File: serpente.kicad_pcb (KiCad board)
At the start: 2 copper layers, 24 x 22 mm, 31 parts, among them J1 USB_C_Receptacle_USB2.0, J2 Conn_Power, J3 Conn_GPIO, SW1 SW_RESET, U1 GD25Q32CNIGR, U2 MCP1700-3302E_SOT23, U3 ATSAMD21E18A

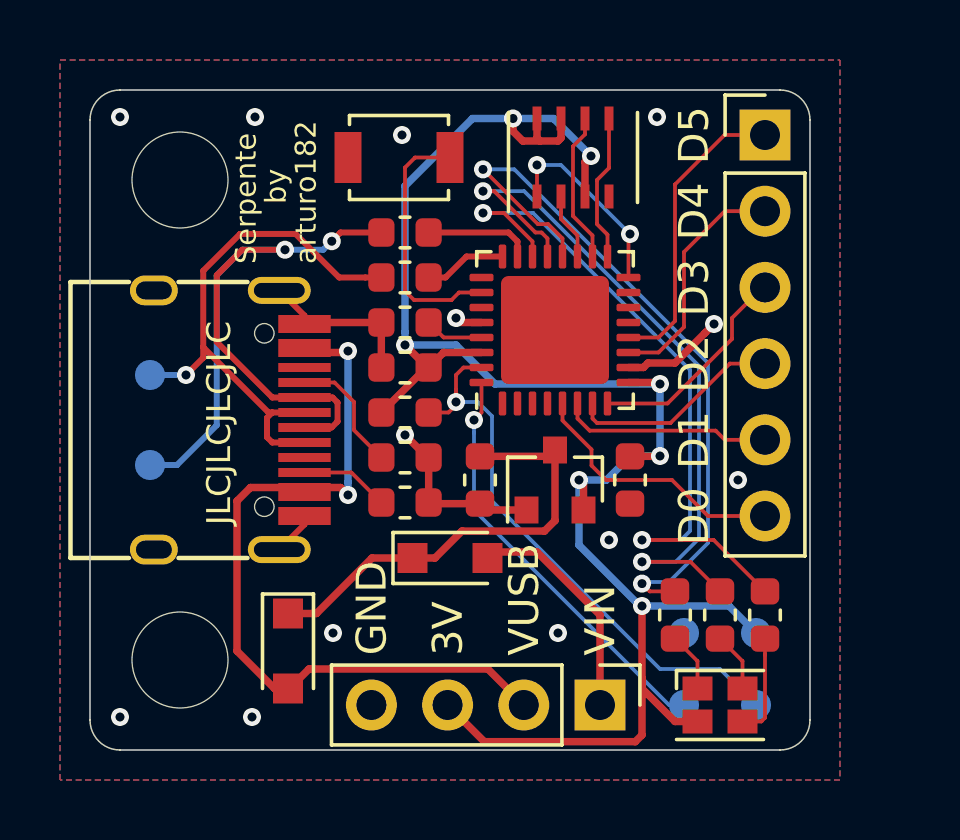
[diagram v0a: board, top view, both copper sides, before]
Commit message: Final rev 2 release!
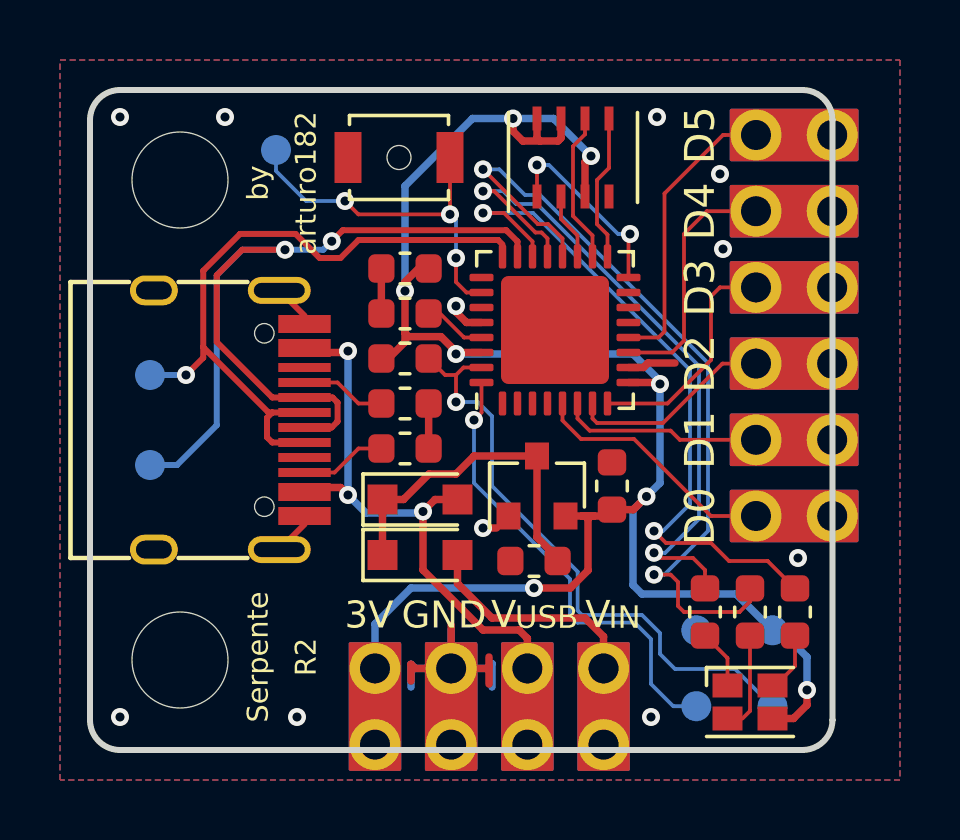
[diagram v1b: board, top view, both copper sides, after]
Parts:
- removed R7, R8: 22R, Resistor_SMD:R_0603_1608Metric
- added TP7: TP_RESET, TestPoint:TestPoint_Pad_D1.0mm, B.Cu at (123.2, 47.0)
- D3: value LED_ARGB -> LED_RBAG
- J2: footprint Connector_PinHeader_2.54mm:PinHeader_1x04_P2.54mm_Vertical -> Connector_PinHeader_2.54mm_Extra:PinHeader_1x04_P2.54mm_Vertical_Castellated
- J3: footprint Connector_PinHeader_2.54mm:PinHeader_1x06_P2.54mm_Vertical -> Connector_PinHeader_2.54mm_Extra:PinHeader_1x06_P2.54mm_Vertical_Castellated
- SW1: footprint Button_Switch_SMD:SW_SPST_B3U-1000P -> Button_Switch_SMD:SW_SPST_B3U-1000P-B
- moved D1 6.70 mm to (128.0, 58.6), turned to 0 degrees
- moved C2 3.30 mm to (127.5, 51.0)
- moved C1 3.24 mm to (131.8, 60.7), turned to 0 degrees
- moved R3 2.50 mm to (140.5, 62.4)
- moved R4 1.80 mm to (127.5, 55.5)
- moved R5 1.80 mm to (127.5, 57.0)
- moved R6 1.80 mm to (127.5, 54.0)
- moved J2 1.23 mm to (134.1, 64.3)
- moved D2 1.00 mm to (128.0, 60.5)
- moved R1 1.00 mm to (137.5, 62.4)
- moved D3 1.00 mm to (139.0, 65.4)
- moved C3 0.63 mm to (134.4, 58.2), turned to 90 degrees
- moved U2 0.63 mm to (131.9, 58.2)
- moved TP3 0.56 mm to (139.8, 63.0)
- moved TP1 0.55 mm to (139.8, 65.5)
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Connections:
- net Net-(SW1-Pad2) renamed /~RESET~
- D3 pad 3: Net-(D3-Pad3) -> +3V3
- D3 pad 4: +3V3 -> Net-(D3-Pad4)
- J2 pad 3: +3V3 -> GND
- J2 pad 4: GND -> +3V3
- R2 pad 1: Net-(D3-Pad3) -> Net-(D3-Pad4)
- U3 pad 20: /LED_R -> /LED_G
- U3 pad 21: /LED_B -> /LED_R
- U3 pad 22: /LED_G -> /LED_B
- U3 pad 23: Net-(R7-Pad1) -> /USB_D-
- U3 pad 24: Net-(R8-Pad1) -> /USB_D+
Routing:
- net GND: track 17.8 -> 23.1 mm, vias 13 -> 11
- net /USB_D-: track 25.4 -> 30.6 mm
- net VBUS: track 26.7 -> 22.3 mm, vias 2 -> 3
- net /USB_D+: track 18.5 -> 22.5 mm
- net +5V: track 15.1 -> 11.3 mm
- net /~RESET~: track 8.53 -> 12.3 mm, vias 0 -> 3
- net /LED_G: track 23.5 -> 27.1 mm
- net Net-(R7-Pad1): track 3.59 -> 0.00 mm
- net Net-(D3-Pad3): track 3.44 -> 0.00 mm
- net /GPIO4: track 7.97 -> 10.8 mm
- net Net-(D3-Pad4): track 0.00 -> 2.87 mm
- net /GPIO3: track 7.26 -> 10.1 mm
- net Net-(R8-Pad1): track 2.75 -> 0.00 mm
- net VIN: track 7.62 -> 9.98 mm
- net /GPIO5: track 10.0 -> 12.3 mm
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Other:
- board size 24 x 22 mm -> 24.8 x 22 mm
- board text added: "CLK"
- board text added: "DAT"
- board text added: "IN"
- board text added: "R2"
- board text added: "RST"
- board text added: "USB"
- board text added: "V"
- board text removed: "C"
- board text removed: "G"
- board text removed: "JLCJLCJLCJLC"
- board text removed: "VIN"
- board text removed: "VUSB"
